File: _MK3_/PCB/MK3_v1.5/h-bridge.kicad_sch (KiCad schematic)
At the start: 14 parts, among them IC1 DRV8874PWPR, IC2 DRV8874PWPR, J10 Conn_01x04_Pin

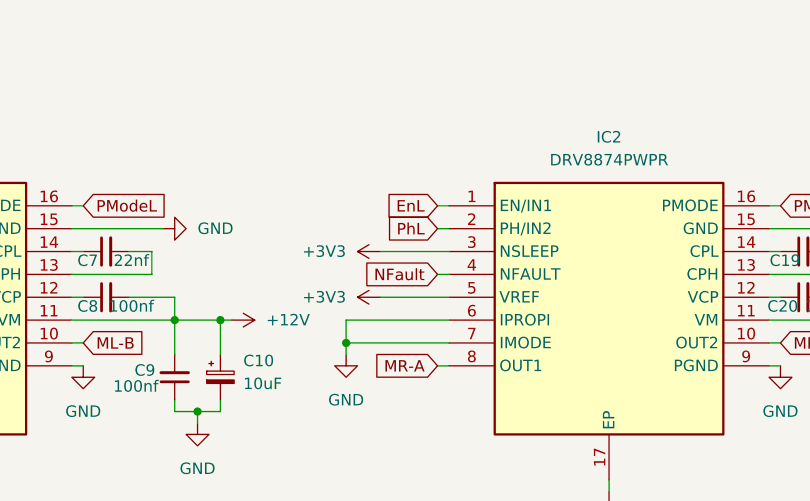
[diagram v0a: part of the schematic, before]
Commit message: pcb done
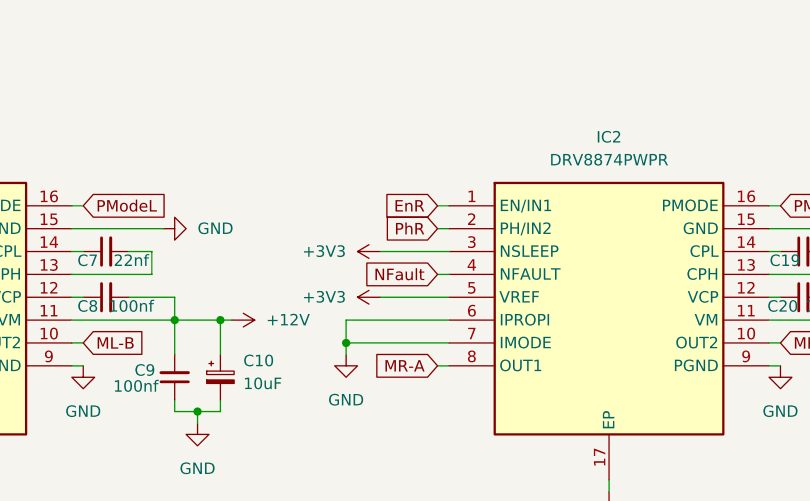
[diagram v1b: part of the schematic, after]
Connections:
- net EnL: no longer IC2.1 (EN/IN1)
- net PhL: no longer IC2.2 (PH/IN2)
- new net EnR: IC2.1 (EN/IN1)
- new net PhR: IC2.2 (PH/IN2)
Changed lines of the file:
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@@
 		)
 	)
-	(global_label "PhL"
+	(global_label "PhR"
 		(shape input)
 		(at 139.7 49.53 180)
@@
 		)
 		(property "Intersheetrefs" "${INTERSHEET_REFS}"
-			(at 133.8192 49.53 0)
+			(at 133.679 49.53 0)
 			(effects
 				(font
@@
 		)
 	)
-	(global_label "EnL"
+	(global_label "EnR"
 		(shape input)
 		(at 139.7 46.99 180)
@@
 		)
 		(property "Intersheetrefs" "${INTERSHEET_REFS}"
-			(at 133.8639 46.99 0)
+			(at 133.7237 46.99 0)
 			(effects
 				(font
